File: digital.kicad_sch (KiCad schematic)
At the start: 36 parts

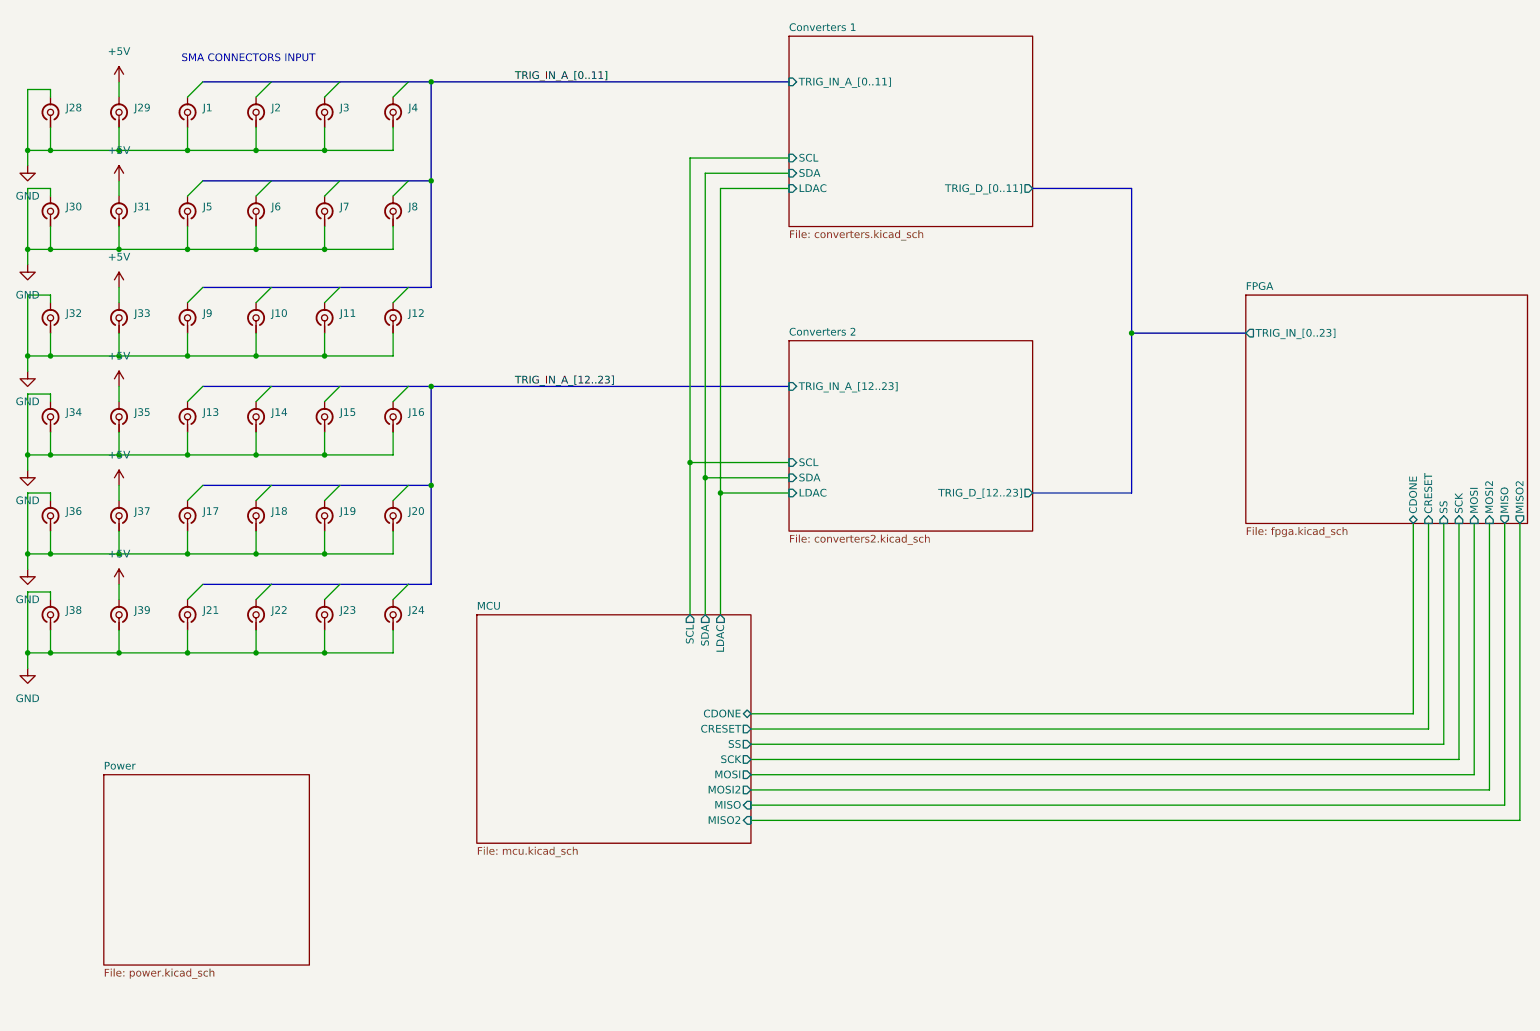
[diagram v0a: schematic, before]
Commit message: Small aesthetic changes and small rework of power sheet.
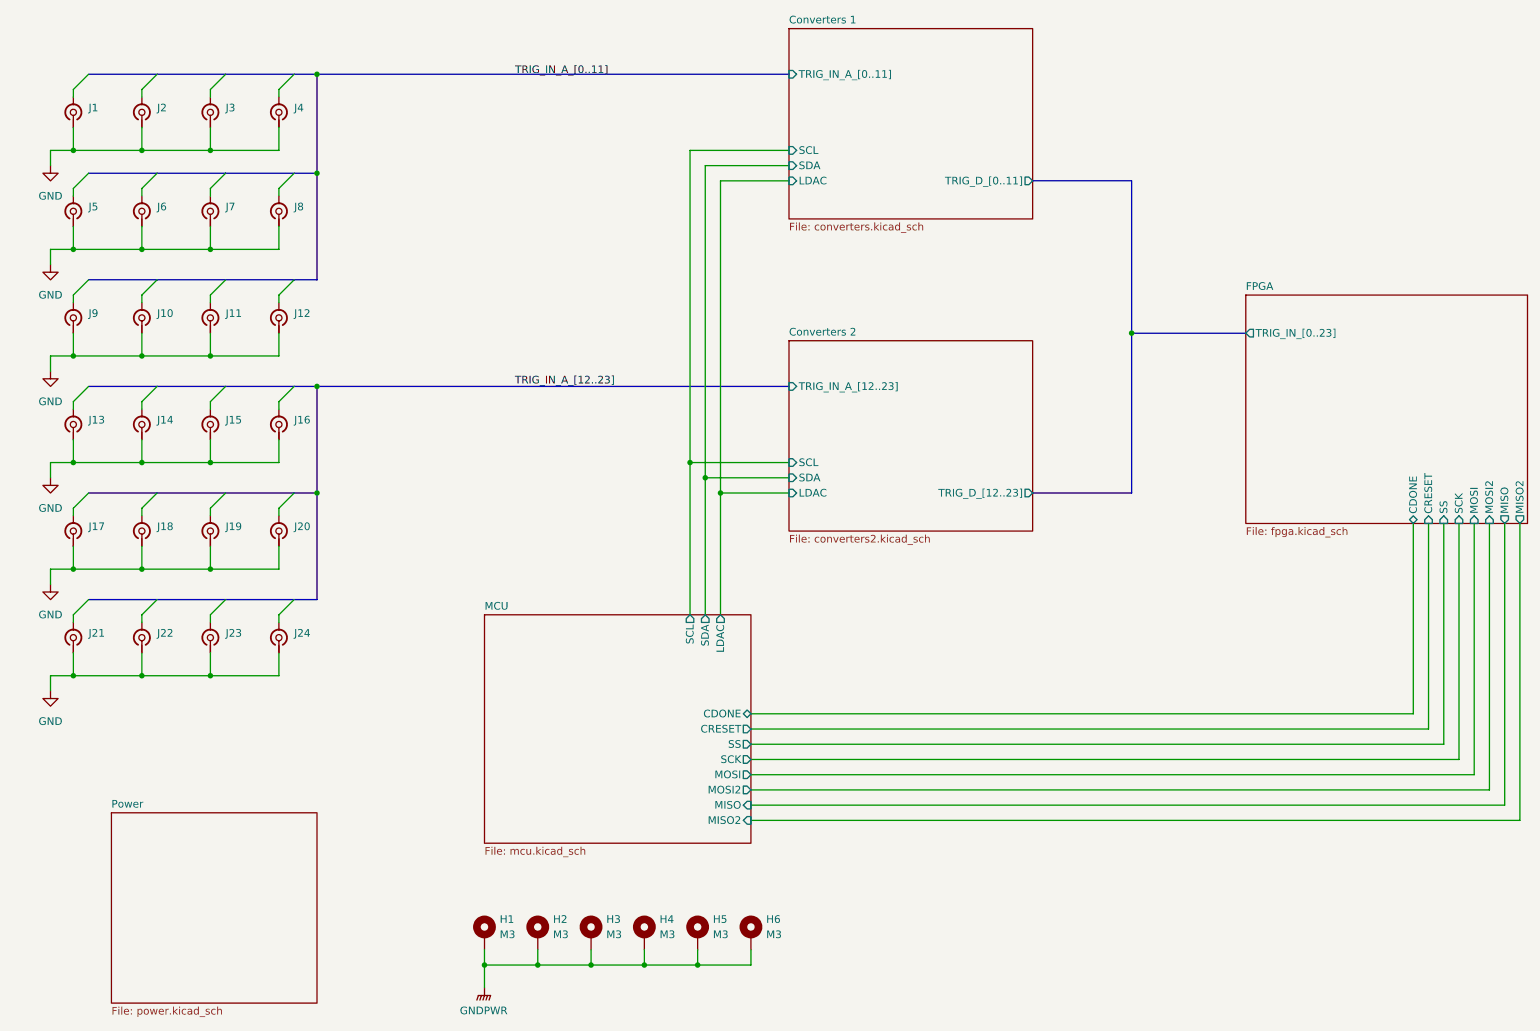
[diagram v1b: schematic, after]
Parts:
- removed J28, J29, J30, J31, J32, J33, J34, J35, J36, J37, J38, J39: ~, symbol Connector:Conn_Coaxial_Small
- added H1, H2, H3, H4, H5, H6: M3, symbol Mechanical:MountingHole_Pad
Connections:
- new net GNDPWR: H1.1, H2.1, H3.1, H4.1, H5.1, H6.1
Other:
- note removed: "SMA CONNECTORS INPUT"
- moved on the sheet: J1, J10, J11, J12, J13, J14, J15, J16, J17, J18, J19, J2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

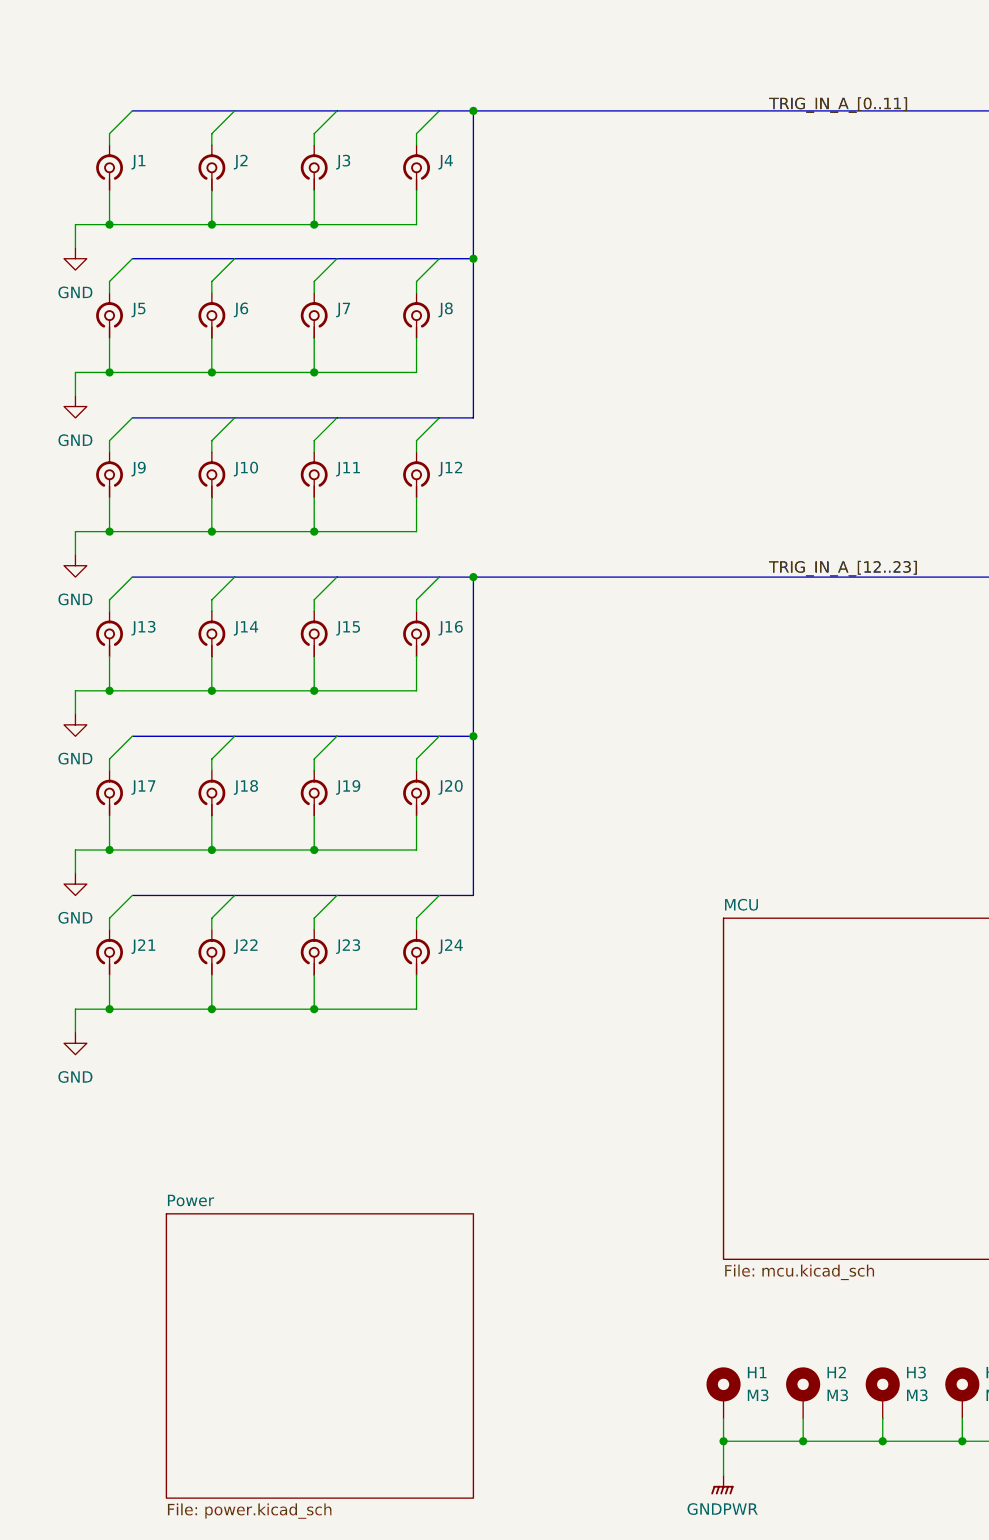
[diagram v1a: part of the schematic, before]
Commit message: complete power
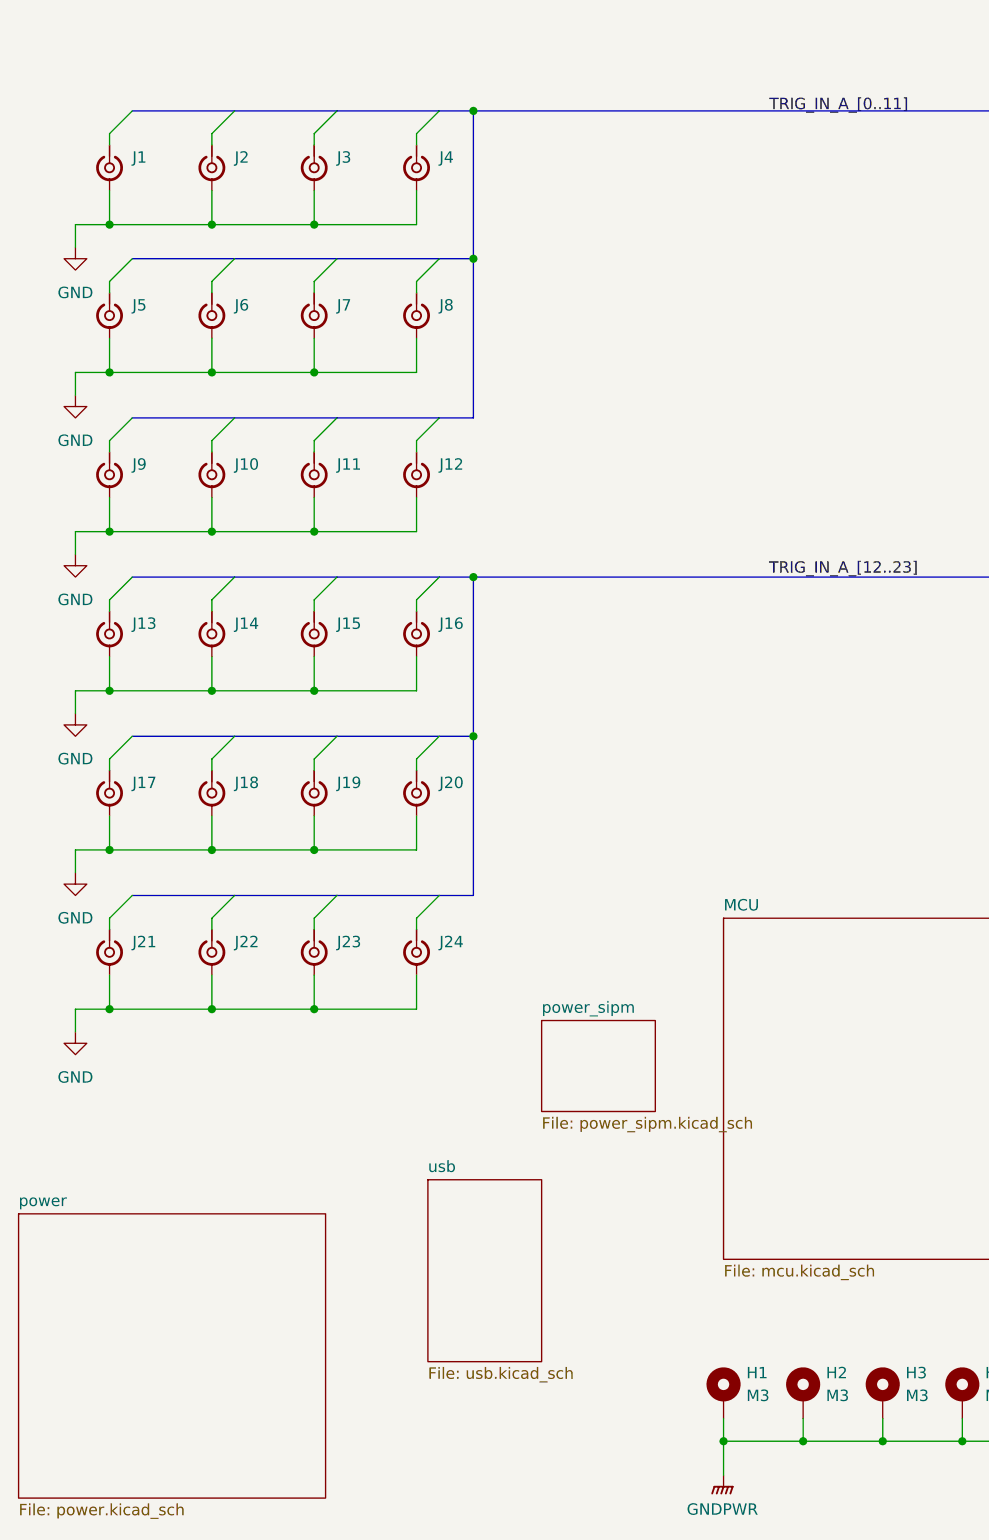
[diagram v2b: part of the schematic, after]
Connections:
- net GND: now also J1.2 (Ext), J10.2 (Ext), J11.2 (Ext), J12.2 (Ext), J13.2 (Ext), J14.2 (Ext), J15.2 (Ext), J16.2 (Ext), J17.2 (Ext), J18.2 (Ext), J19.2 (Ext), J2.2 (Ext), J20.2 (Ext), J21.2 (Ext), J22.2 (Ext), J23.2 (Ext), J24.2 (Ext), J3.2 (Ext), J4.2 (Ext), J5.2 (Ext), J6.2 (Ext), J7.2 (Ext), J8.2 (Ext), J9.2 (Ext); no longer J1.1 (In), J10.1 (In), J11.1 (In), J12.1 (In), J13.1 (In), J14.1 (In), J15.1 (In), J16.1 (In), J17.1 (In), J18.1 (In), J19.1 (In), J2.1 (In), J20.1 (In), J21.1 (In), J22.1 (In), J23.1 (In), J24.1 (In), J3.1 (In), J4.1 (In), J5.1 (In), J6.1 (In), J7.1 (In), J8.1 (In), J9.1 (In)
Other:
- sheet Power renamed power
- added sheet power_sipm (power_sipm.kicad_sch)
- added sheet usb (usb.kicad_sch)
- moved on the sheet: J1, J10, J11, J12, J13, J14, J15, J16, J17, J18, J19, J2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
